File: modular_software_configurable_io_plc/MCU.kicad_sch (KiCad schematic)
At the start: 2 parts, among them J32 FW-41-03-G-D-085-155

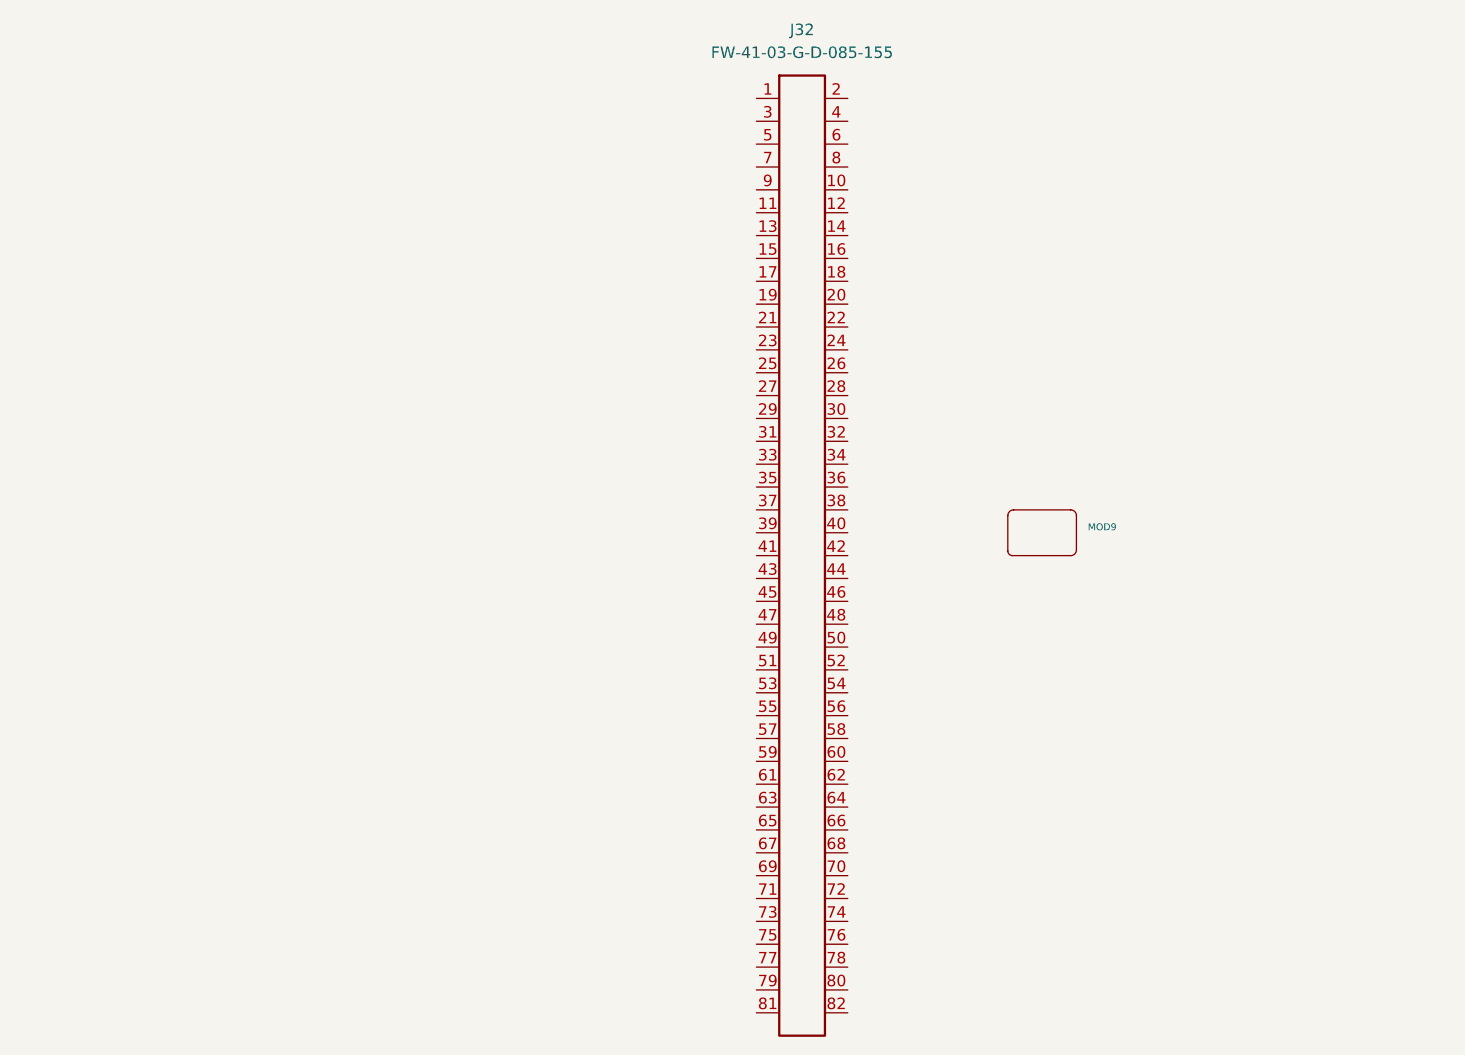
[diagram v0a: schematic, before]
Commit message: development backup
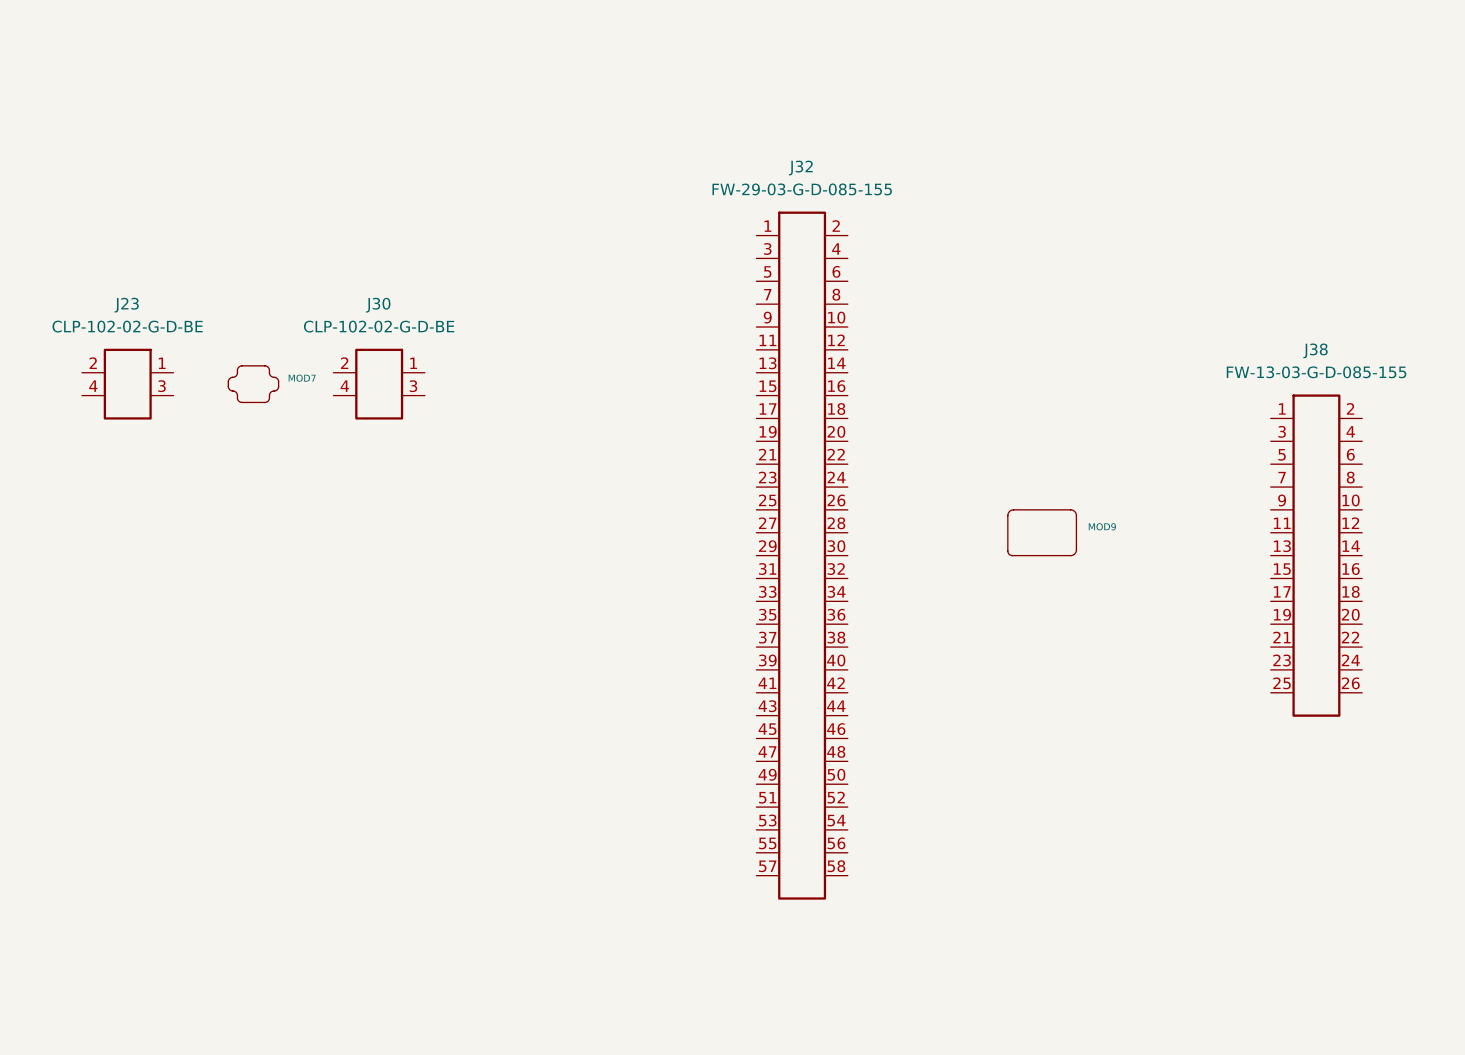
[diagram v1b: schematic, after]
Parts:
- added J23, J30: CLP-102-02-G-D-BE, connector_footprints:CLP-102-02-G-D-BE, symbol UNITED_CONNECTORS_DATA_BASE:J_CLP-102-02-G-D-BE
- added J38: FW-13-03-G-D-085-155, connector_footprints:FW-13-03-G-D-085-155, symbol UNITED_CONNECTORS_DATA_BASE:J_FW-13-03-G-D-085-155
- added MOD7: ~, modules_footprints:minimal_max17761, symbol UNITED_MODULES_DATA_BASE:MINIMAL_MAX17761
- J32: value FW-41-03-G-D-085-155 -> FW-29-03-G-D-085-155; footprint connector_footprints:FW-41-03-G-D-085-155 -> connector_footprints:FW-29-03-G-D-085-155; symbol UNITED_CONNECTORS_DATA_BASE:J_FW-41-03-G-D-085-155 -> UNITED_CONNECTORS_DATA_BASE:J_FW-29-03-G-D-085-155; MPN FW-41-03-G-D-085-155 -> FW-29-03-G-D-085-155; Pin Count 41 -> 29; Symbol Name J_FW-41-03-G-D-085-155 -> J_FW-29-03-G-D-085-155; Trustedparts Search https://www.trustedparts.com/en/search/FW-41-03-G-D-085-155 -> https://www.trustedparts.com/en/search/FW-29-03-G-D-085-155

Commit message: Backup
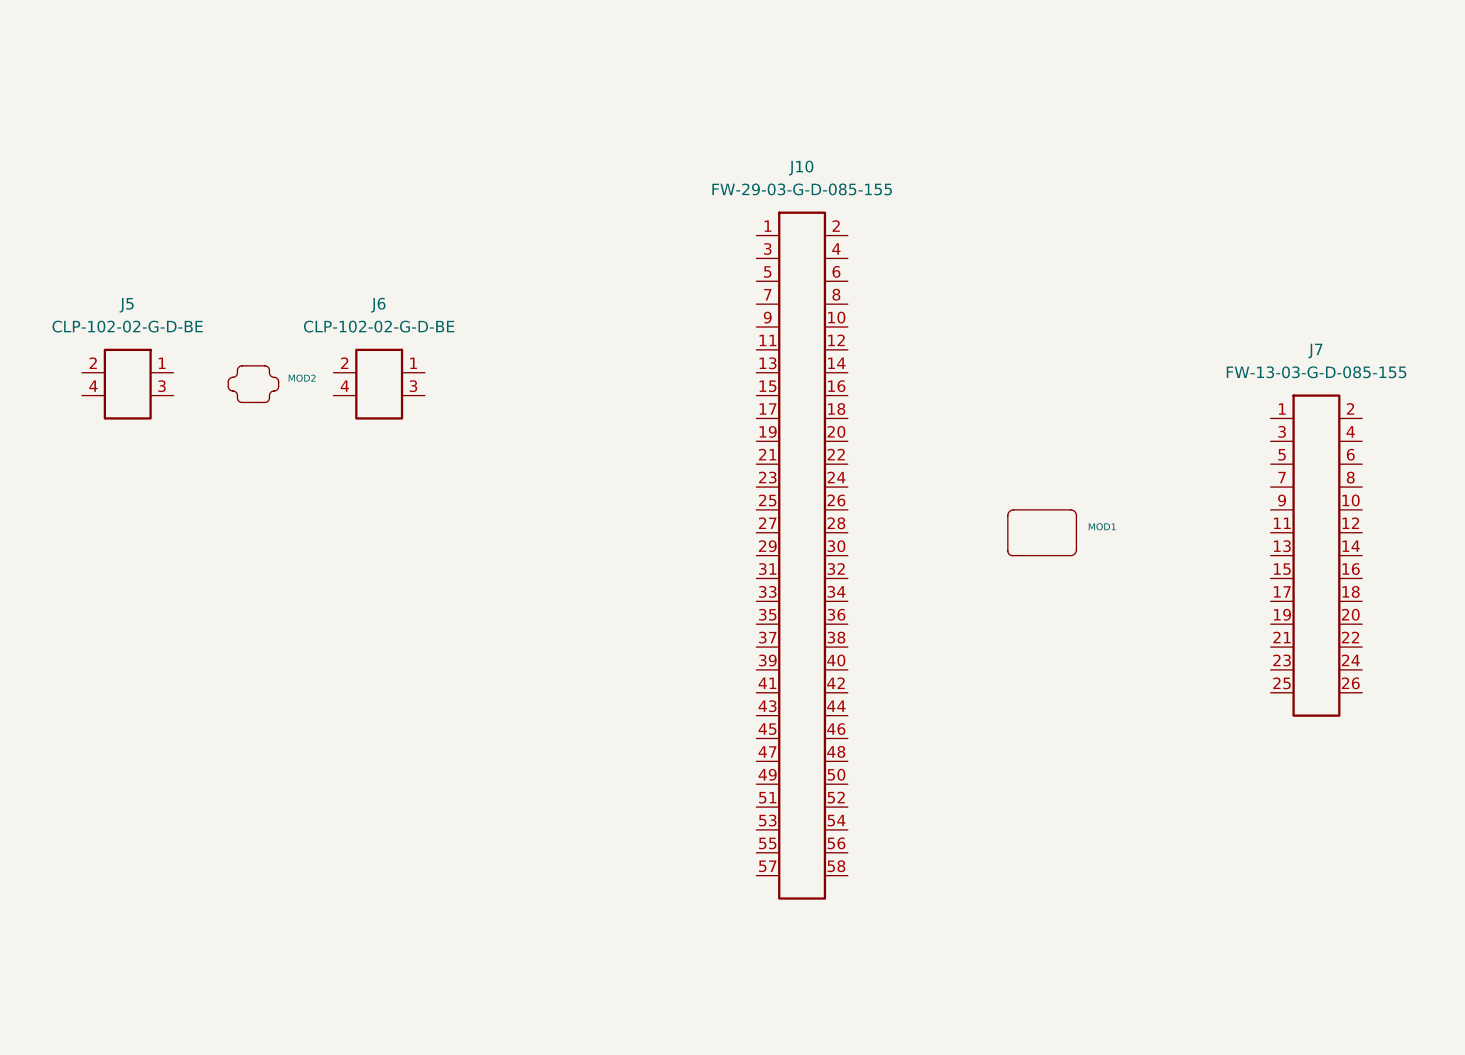
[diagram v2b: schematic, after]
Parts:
- renumbered J32 to J10, J23 to J5, J30 to J6, J38 to J7, MOD9 to MOD1, MOD7 to MOD2
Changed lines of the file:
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@@
 		(dnp no)
 		(fields_autoplaced yes)
-		(property "Reference" "MOD9"
+		(property "Reference" "MOD1"
 			(at 147.32 104.776 0)
 			(effects
@@
 			(project ""
 				(path "/b764ffe3-5231-4422-b46d-b0de4c44c7b4/1ba52bb1-dfa5-4e79-b99c-b54242d8ec88"
-					(reference "MOD9")
+					(reference "MOD1")
 					(unit 1)
 				)
@@
 		(dnp no)
 		(fields_autoplaced yes)
-		(property "Reference" "J23"
+		(property "Reference" "J5"
 			(at 40.64 80.01 0)
 			(effects
@@
 			(project "modular_software_configurable_io_plc"
 				(path "/b764ffe3-5231-4422-b46d-b0de4c44c7b4/1ba52bb1-dfa5-4e79-b99c-b54242d8ec88"
-					(reference "J23")
+					(reference "J5")
 					(unit 1)
 				)
@@
 		(dnp no)
 		(fields_autoplaced yes)
-		(property "Reference" "J38"
+		(property "Reference" "J7"
 			(at 172.72 85.09 0)
 			(effects
@@
 			(project "modular_software_configurable_io_plc"
 				(path "/b764ffe3-5231-4422-b46d-b0de4c44c7b4/1ba52bb1-dfa5-4e79-b99c-b54242d8ec88"
-					(reference "J38")
+					(reference "J7")
 					(unit 1)
 				)
@@
 		(dnp no)
 		(fields_autoplaced yes)
-		(property "Reference" "MOD7"
+		(property "Reference" "MOD2"
 			(at 58.42 88.265 0)
 			(effects
@@
 			(project "modular_software_configurable_io_plc"
 				(path "/b764ffe3-5231-4422-b46d-b0de4c44c7b4/1ba52bb1-dfa5-4e79-b99c-b54242d8ec88"
-					(reference "MOD7")
+					(reference "MOD2")
 					(unit 1)
 				)
@@
 		(dnp no)
 		(fields_autoplaced yes)
-		(property "Reference" "J30"
+		(property "Reference" "J6"
 			(at 68.58 80.01 0)
 			(effects
@@
 			(project "modular_software_configurable_io_plc"
 				(path "/b764ffe3-5231-4422-b46d-b0de4c44c7b4/1ba52bb1-dfa5-4e79-b99c-b54242d8ec88"
-					(reference "J30")
+					(reference "J6")
 					(unit 1)
 				)
@@
 		(dnp no)
 		(fields_autoplaced yes)
-		(property "Reference" "J32"
+		(property "Reference" "J10"
 			(at 115.57 64.77 0)
 			(effects
@@
 			(project "modular_software_configurable_io_plc"
 				(path "/b764ffe3-5231-4422-b46d-b0de4c44c7b4/1ba52bb1-dfa5-4e79-b99c-b54242d8ec88"
-					(reference "J32")
+					(reference "J10")
 					(unit 1)
 				)
